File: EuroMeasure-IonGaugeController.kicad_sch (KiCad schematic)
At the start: 5 parts

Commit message: Rename to Ion Gauge Controller
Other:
- title: EuroMeasure blank module -> EuroMeasure Ion Gauge Controller
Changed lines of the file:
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@@
   (paper "A4")
   (title_block
-    (title "EuroMeasure blank module")
+    (title "EuroMeasure Ion Gauge Controller")
+    (date "2023-10-17")
+    (rev "1.0.0")
   )
   (bus_alias "ADC_ISO" (members "RESET" "DRDY" "CS" "SCLK" "DIN" "DOUT" "CLK"))
@@
     (pin "1")
     (instances
-      (project "EuroMeasure-Module"
+      (project "EuroMeasure-IonGaugeController"
         (path "/9c84a828-ebcc-4f88-b5cc-11be4f5044ad/abf38db6-df21-42a4-a2d8-4fd7d247b99e"
           (reference "TP909") (unit 1)
@@
     (pin "1")
     (instances
-      (project "EuroMeasure-Module"
+      (project "EuroMeasure-IonGaugeController"
         (path "/9c84a828-ebcc-4f88-b5cc-11be4f5044ad/abf38db6-df21-42a4-a2d8-4fd7d247b99e"
           (reference "TP908") (unit 1)
@@
     (pin "1")
     (instances
-      (project "EuroMeasure-Module"
+      (project "EuroMeasure-IonGaugeController"
         (path "/9c84a828-ebcc-4f88-b5cc-11be4f5044ad/abf38db6-df21-42a4-a2d8-4fd7d247b99e"
           (reference "TP910") (unit 1)
@@
     (pin "1")
     (instances
-      (project "EuroMeasure-Module"
+      (project "EuroMeasure-IonGaugeController"
         (path "/9c84a828-ebcc-4f88-b5cc-11be4f5044ad/abf38db6-df21-42a4-a2d8-4fd7d247b99e"
           (reference "TP906") (unit 1)
@@
     (pin "1")
     (instances
-      (project "EuroMeasure-Module"
+      (project "EuroMeasure-IonGaugeController"
         (path "/9c84a828-ebcc-4f88-b5cc-11be4f5044ad/abf38db6-df21-42a4-a2d8-4fd7d247b99e"
           (reference "TP907") (unit 1)
@@
     )
     (instances
-      (project "EuroMeasure-Module"
+      (project "EuroMeasure-IonGaugeController"
         (path "/9c84a828-ebcc-4f88-b5cc-11be4f5044ad" (page "3"))
       )

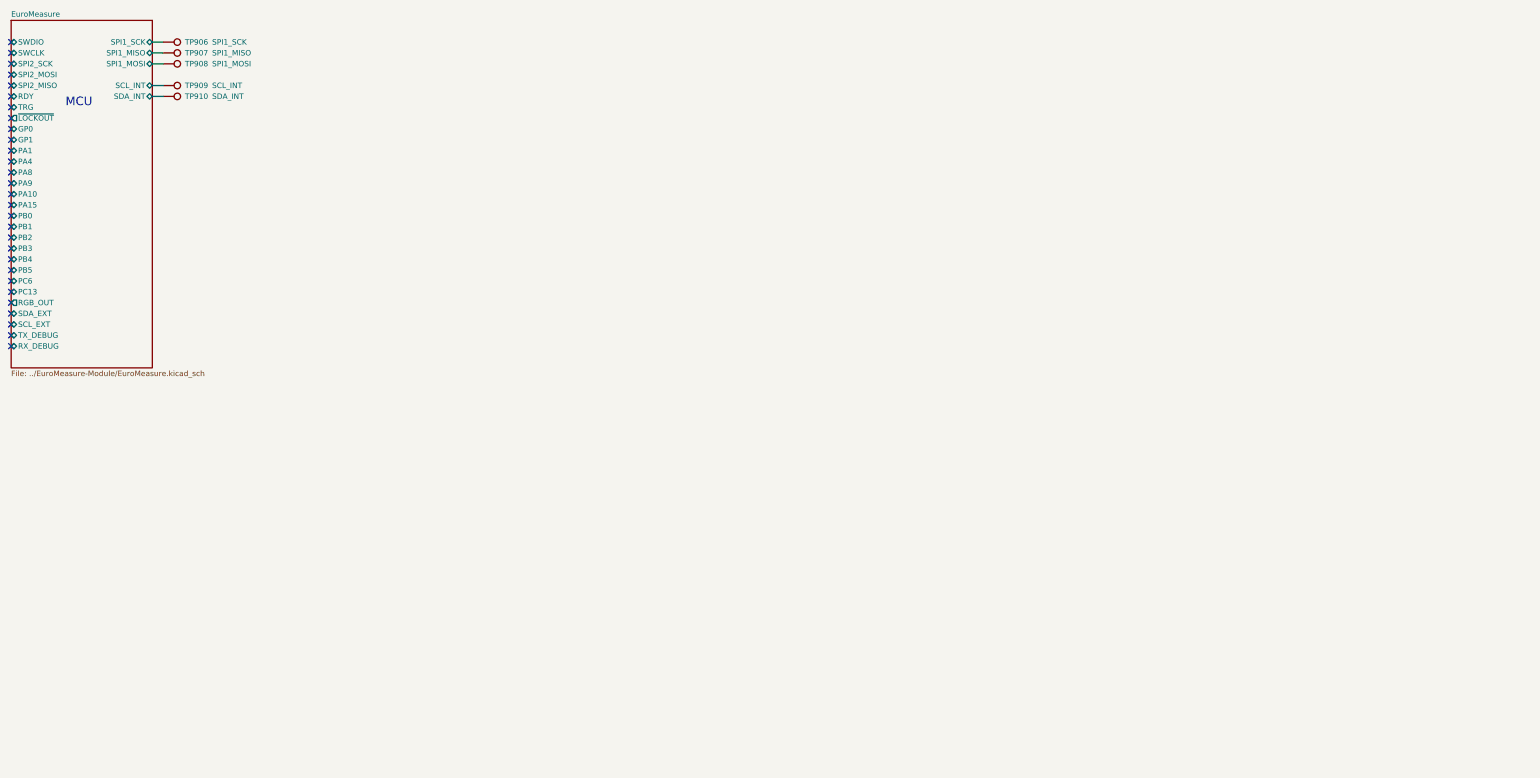
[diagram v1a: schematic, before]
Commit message: First schematic draft
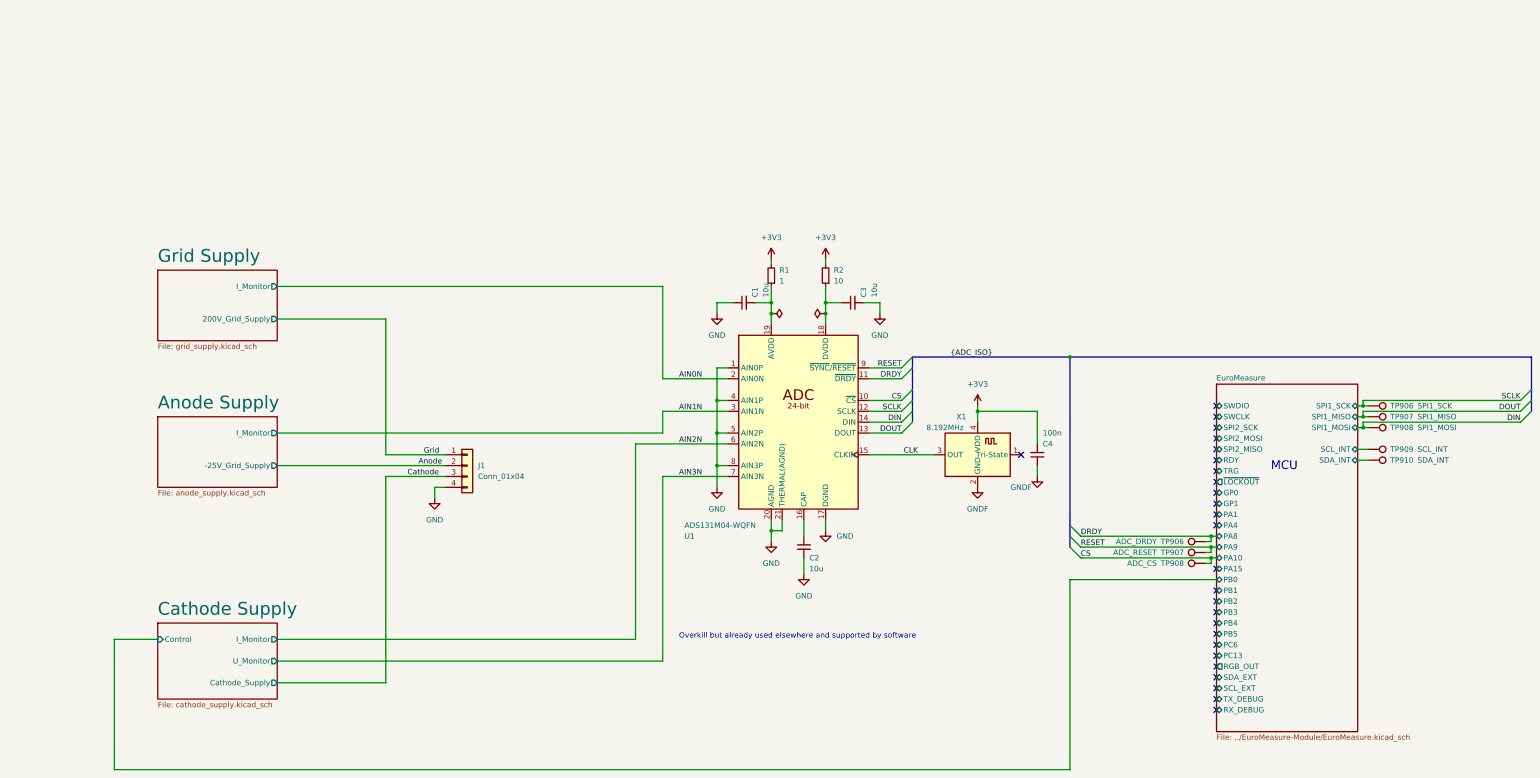
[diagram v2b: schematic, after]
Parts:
- added C1, C2, C3: 10u, Capacitor_SMD:C_0805_2012Metric_Pad1.18x1.45mm_HandSolder, symbol Device:C_Small
- added C4: 100n, Capacitor_SMD:C_0805_2012Metric_Pad1.18x1.45mm_HandSolder, symbol Device:C_Small
- added J1: Conn_01x04, symbol Connector_Generic:Conn_01x04
- added R1: 1, Resistor_SMD:R_0805_2012Metric_Pad1.20x1.40mm_HandSolder, symbol Device:R_Small
- added R2: 10, Resistor_SMD:R_0805_2012Metric_Pad1.20x1.40mm_HandSolder, symbol Device:R_Small
- added TP906: ADC_DRDY, MEMS_Custom:TestPoint_Pad_D1.0mm, symbol Connector:TestPoint
- added TP907: ADC_RESET, MEMS_Custom:TestPoint_Pad_D1.0mm, symbol Connector:TestPoint
- added TP908: ADC_CS, MEMS_Custom:TestPoint_Pad_D1.0mm, symbol Connector:TestPoint
- added U1: ADS131M04-WQFN, Package_DFN_QFN:WQFN-20-1EP_3x3mm_P0.4mm_EP1.7x1.7mm, symbol MEMS_IC:ADS131M04-WQFN
- added X1: 8.192MHz, Oscillator:Oscillator_SMD_ECS_2520MV-xxx-xx-4Pin_2.5x2.0mm, symbol MEMS_IC:ECS-2520MVLC-081.92-CN-TR_oscillator_8.192MHZ
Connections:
- net EuroMeasure/SPI1_MISO renamed DOUT
- net DOUT: now also U1.13 (DOUT)
- net EuroMeasure/SPI1_MOSI renamed DIN
- net DIN: now also U1.14 (DIN)
- net EuroMeasure/SPI1_SCK renamed SCLK
- net SCLK: now also U1.12 (SCLK)
- new net: C3.1, R2.1, U1.18 (DVDD)
- new net: C1.2, R1.1, U1.19 (AVDD)
- new net: C2.1, U1.16 (CAP)
- new net +3V3: C4.2, R1.2, R2.2, X1.4 (VDD)
- new net AIN0N: U1.2 (AIN0N)
- new net AIN1N: U1.3 (AIN1N)
- new net AIN2N: U1.6 (AIN2N)
- new net AIN3N: U1.7 (AIN3N)
- new net Anode: J1.2 (Pin_2)
- new net CLK: U1.15 (CLKIN), X1.3 (OUT)
- new net CS: TP908.1, U1.10 (~{CS})
- new net Cathode: J1.3 (Pin_3)
- new net DRDY: TP906.1, U1.11 (~{DRDY})
- new net GND: C1.1, C2.2, C3.2, J1.4 (Pin_4), U1.1 (AIN0P), U1.17 (DGND), U1.20 (AGND), U1.21 (THERMAL(AGND)), U1.4 (AIN1P), U1.5 (AIN2P), U1.8 (AIN3P)
- new net GNDF: C4.1, X1.2 (GND)
- new net Grid: J1.1 (Pin_1)
- new net RESET: TP907.1, U1.9 (~{SYNC}/~{RESET})
- no-connect marks 29 -> 26
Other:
- added sheet Anode Supply (anode_supply.kicad_sch)
- added sheet Cathode Supply (cathode_supply.kicad_sch)
- added sheet Grid Supply (grid_supply.kicad_sch)
- note added: "Overkill but already used elsewhere and supported by software"
- moved on the sheet: TP906, TP907, TP908, TP909, TP910
